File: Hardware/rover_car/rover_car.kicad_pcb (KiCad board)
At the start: 2 copper layers, 36.8 x 71.1 mm, 29 parts, among them J1 Conn_01x06_Female, J3 Screw_Terminal_01x02, M1 Motor_DC, M2 Motor_DC, M3 Motor_DC, M4 Motor_DC, M5 Motor_DC, M6 Motor_DC, U1 DRV8833PWP, U2 DRV8833PWP, U3 DRV8833PWP

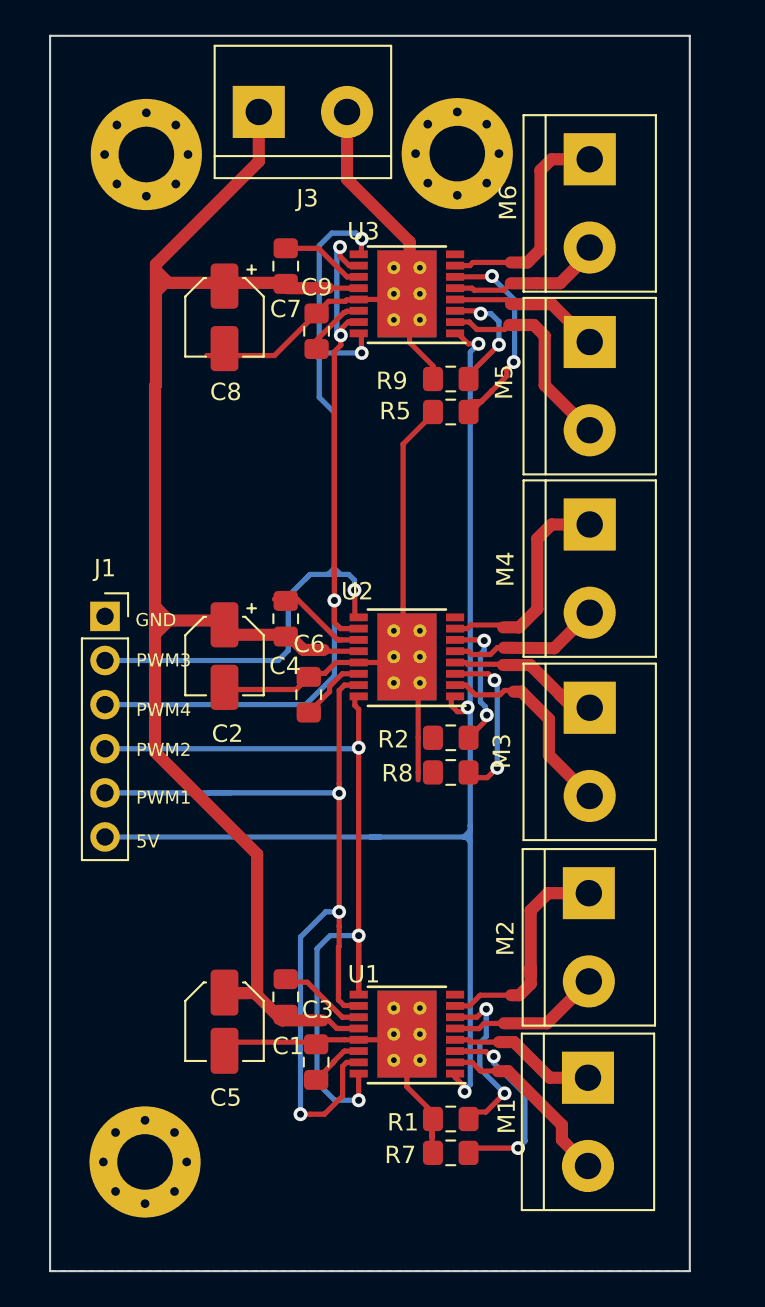
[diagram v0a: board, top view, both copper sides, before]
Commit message: Last revision pcb
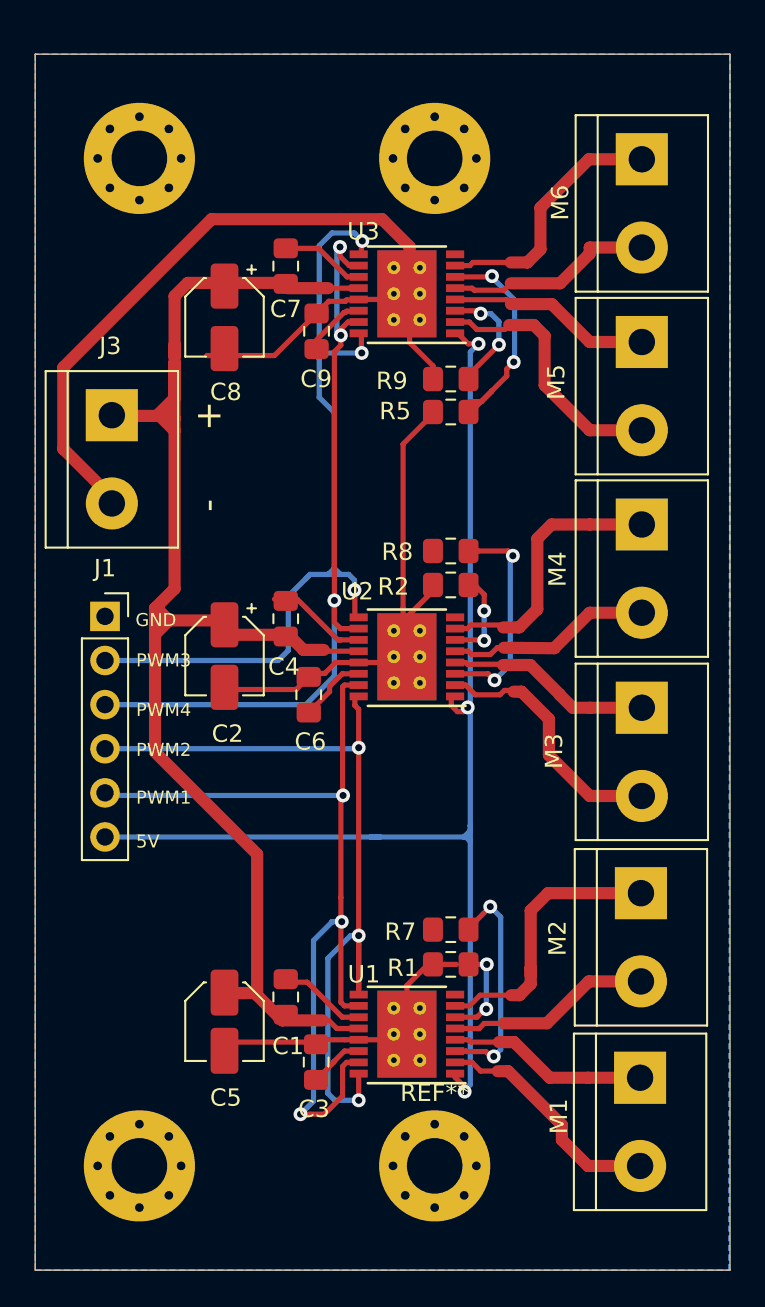
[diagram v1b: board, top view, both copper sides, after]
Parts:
- added REF**: MountingHole_3.2mm_M3_Pad_Via, MountingHole:MountingHole_3.2mm_M3_Pad_Via, F.Cu at (156.0, 93.0)
- moved J3 19.4 mm to (137.4, 49.8), turned to 270 degrees
- moved R7 12.8 mm to (156.9, 79.4)
- moved R8 12.7 mm to (156.9, 57.6)
- moved R1 8.90 mm to (156.9, 81.4)
- moved R2 8.80 mm to (156.9, 59.6)
- moved M1 3.00 mm to (167.8, 87.9)
- moved M2 3.00 mm to (167.9, 77.3)
- moved M3 3.00 mm to (167.9, 66.6)
- moved M4 3.00 mm to (167.9, 56.1)
- moved M5 3.00 mm to (167.9, 45.6)
- moved M6 3.00 mm to (167.9, 35.0)
- moved REF** 1.33 mm to (156.0, 35.0)
- moved REF** 0.46 mm to (139.0, 35.0)
- moved REF** 0.40 mm to (139.0, 93.0)
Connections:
- net /GPIO2 renamed /GPIO12
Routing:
- net GND: track 89.2 -> 109.6 mm
- net +12V: track 92.7 -> 86.2 mm
- net Net-(R1-Pad1): track 10.2 -> 5.63 mm
- net Net-(R8-Pad1): track 9.76 -> 13.0 mm
- net /BOUT2: track 8.83 -> 11.8 mm
- net /BOUT1: track 13.3 -> 16.3 mm
- net /BFDER2: track 9.09 -> 12.1 mm
- net /BFDER1: track 13.5 -> 16.5 mm
- net /AOUT2: track 8.56 -> 11.6 mm
- net /AOUT1: track 10.5 -> 13.5 mm
- net /AFDER2: track 9.89 -> 12.9 mm
- net /AFDER1: track 12.0 -> 15.0 mm
- net /ADER2: track 8.61 -> 11.6 mm
- net /ADER1: track 12.1 -> 15.1 mm
- net /BDER2: track 8.87 -> 11.9 mm
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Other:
- board size 36.8 x 71.1 mm -> 40 x 70 mm
- board text added: "+"
- board text added: "-"
